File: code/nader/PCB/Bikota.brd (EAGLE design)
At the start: 109.2 x 100 mm, 27 parts, among them Q1 IRLML6244

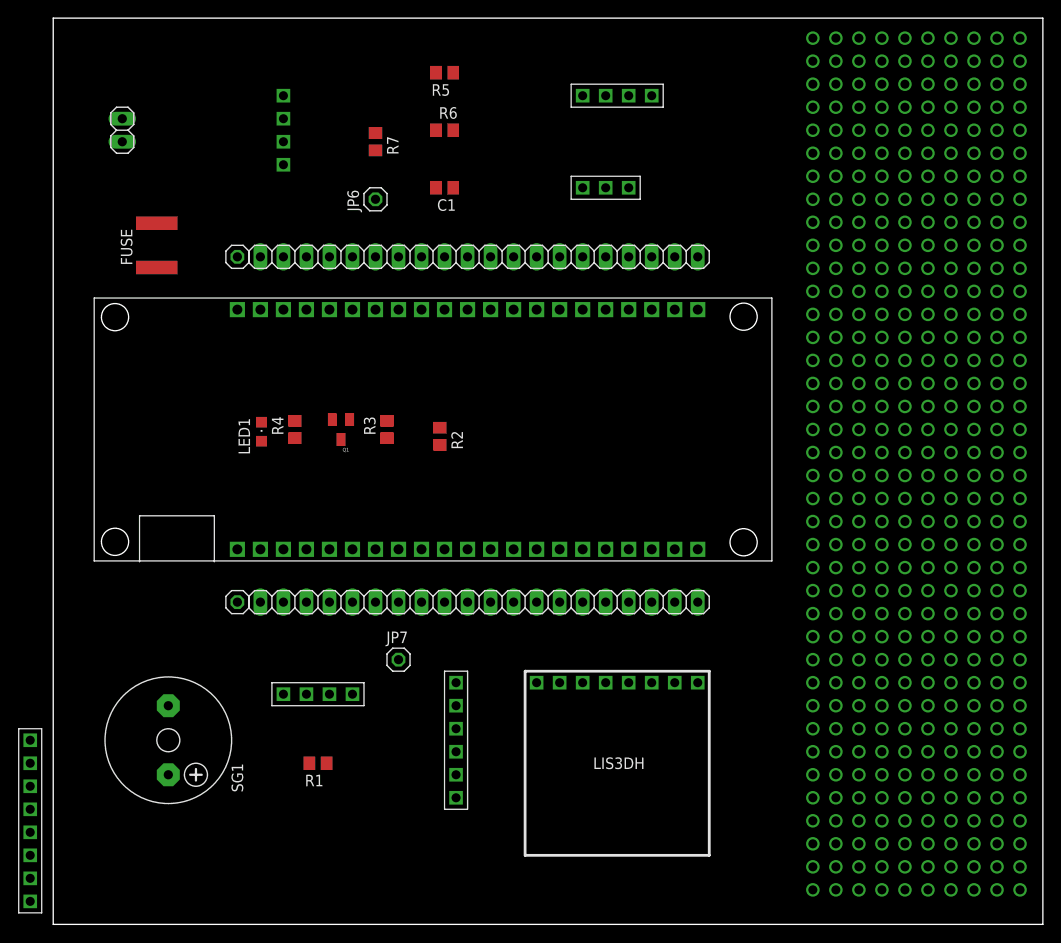
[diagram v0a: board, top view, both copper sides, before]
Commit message: Update PCB and SCH
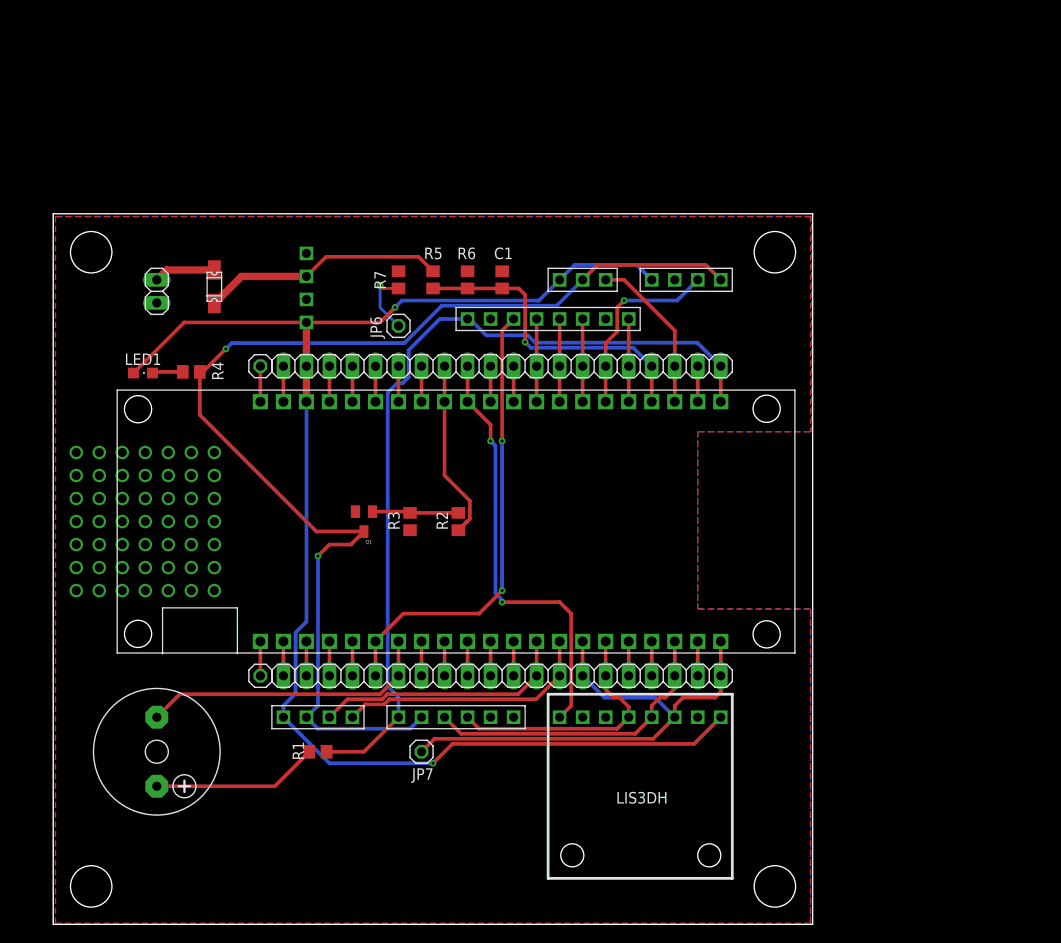
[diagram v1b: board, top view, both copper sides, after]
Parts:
- removed FUSE: MF-SMDF050, fuse:MF-SMDF050
- added F1: 1206L, ptc-littlefuse:1206L
- moved U$7 79.6 mm to (54.6, 66.8), turned to 90 degrees
- moved R5 22.9 mm to (41.9, 71.1), turned to 90 degrees
- moved U$3 21.7 mm to (69.8, 71.1)
- moved JP1 18.2 mm to (11.4, 69.8)
- moved U$8 17.6 mm to (21.6, 70.2)
- moved R6 16.7 mm to (45.7, 71.1), turned to 270 degrees
- moved R7 15.5 mm to (38.1, 71.1)
- moved LED1 14.6 mm to (9.91, 60.8), turned to 270 degrees
- moved JP6 14.2 mm to (38.1, 66.0)
- moved R4 13.1 mm to (15.2, 61.0), turned to 180 degrees
- moved JP2 12.3 mm to (49.5, 61.6)
- moved JP4 12.3 mm to (22.9, 61.6)
- moved C1 12.0 mm to (49.5, 71.1), turned to 90 degrees
- moved JP7 10.5 mm to (40.6, 19.1), turned to 180 degrees
- moved U$1 10.5 mm to (44.5, 44.5)
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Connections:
- removed net N$1: JP2.16, U$1.GPIO34
- removed net N$28: JP3.16, U$1.GPIO15
- removed net N$412: U$7.P$1
- removed net N$413: U$7.P$2
- removed net N$414: U$7.P$3
- removed net N$415: U$7.P$4
- removed net N$416: U$7.P$5
- removed net N$417: U$7.P$6
- removed net N$419: U$7.P$8
- removed net N$5: JP2.14, U$1.GPIO32
- removed net N$7: JP2.13, U$1.GPIO33
- removed net N$8: JP2.12, U$1.GPIO25
- new net EP_BUSY: JP2.16, U$1.GPIO34, U$7.P$8
- new net EP_CLK: JP2.12, U$1.GPIO25, U$7.P$4
- new net EP_CS: JP2.13, U$1.GPIO33, U$7.P$5
- new net EP_DC: JP2.14, U$1.GPIO32, U$7.P$6
- new net EP_DIN: JP3.16, U$1.GPIO15, U$7.P$3
- new net N$41: F1.P$2, JP1.1
- net ESP3V3: now also U$7.P$1
- net GND: now also JP7.1, U$7.P$2
- net VBAT+: now also F1.P$1; no longer JP1.1
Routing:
- net ESP5V: track 0.00 -> 159.9 mm, vias 0 -> 2
- net MOSFET_GND: track 0.00 -> 129.5 mm, vias 0 -> 2
- net ESP3V3: track 0.00 -> 93.8 mm
- net GND: track 0.00 -> 62.6 mm
- net EP_DIN: track 0.00 -> 50.6 mm, vias 0 -> 2
- net ACC_INT: track 0.00 -> 47.7 mm, vias 0 -> 2
- net SVN: track 0.00 -> 34.7 mm, vias 0 -> 1
- net SCL: track 0.00 -> 34.2 mm
- net BUZZER: track 0.00 -> 32.4 mm
- net SDA: track 0.00 -> 28.6 mm
- net PM25: track 0.00 -> 28.5 mm
- net PM10: track 0.00 -> 28.5 mm
- net VBAT+: track 0.00 -> 26.9 mm
- net GPS_TX: track 0.00 -> 21.1 mm, vias 0 -> 1
- net MOSFET: track 0.00 -> 19.8 mm
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- added copper zone on layer 1, net GND
- added copper zone on layer 16, net GND
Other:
- board size 109.2 x 100 mm -> 83.8 x 78.4 mm
